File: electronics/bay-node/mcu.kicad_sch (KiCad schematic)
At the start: 15 parts, among them SW1 RESET, SW2 BOOT, U3 ESP32-S3-MINI-1-N8

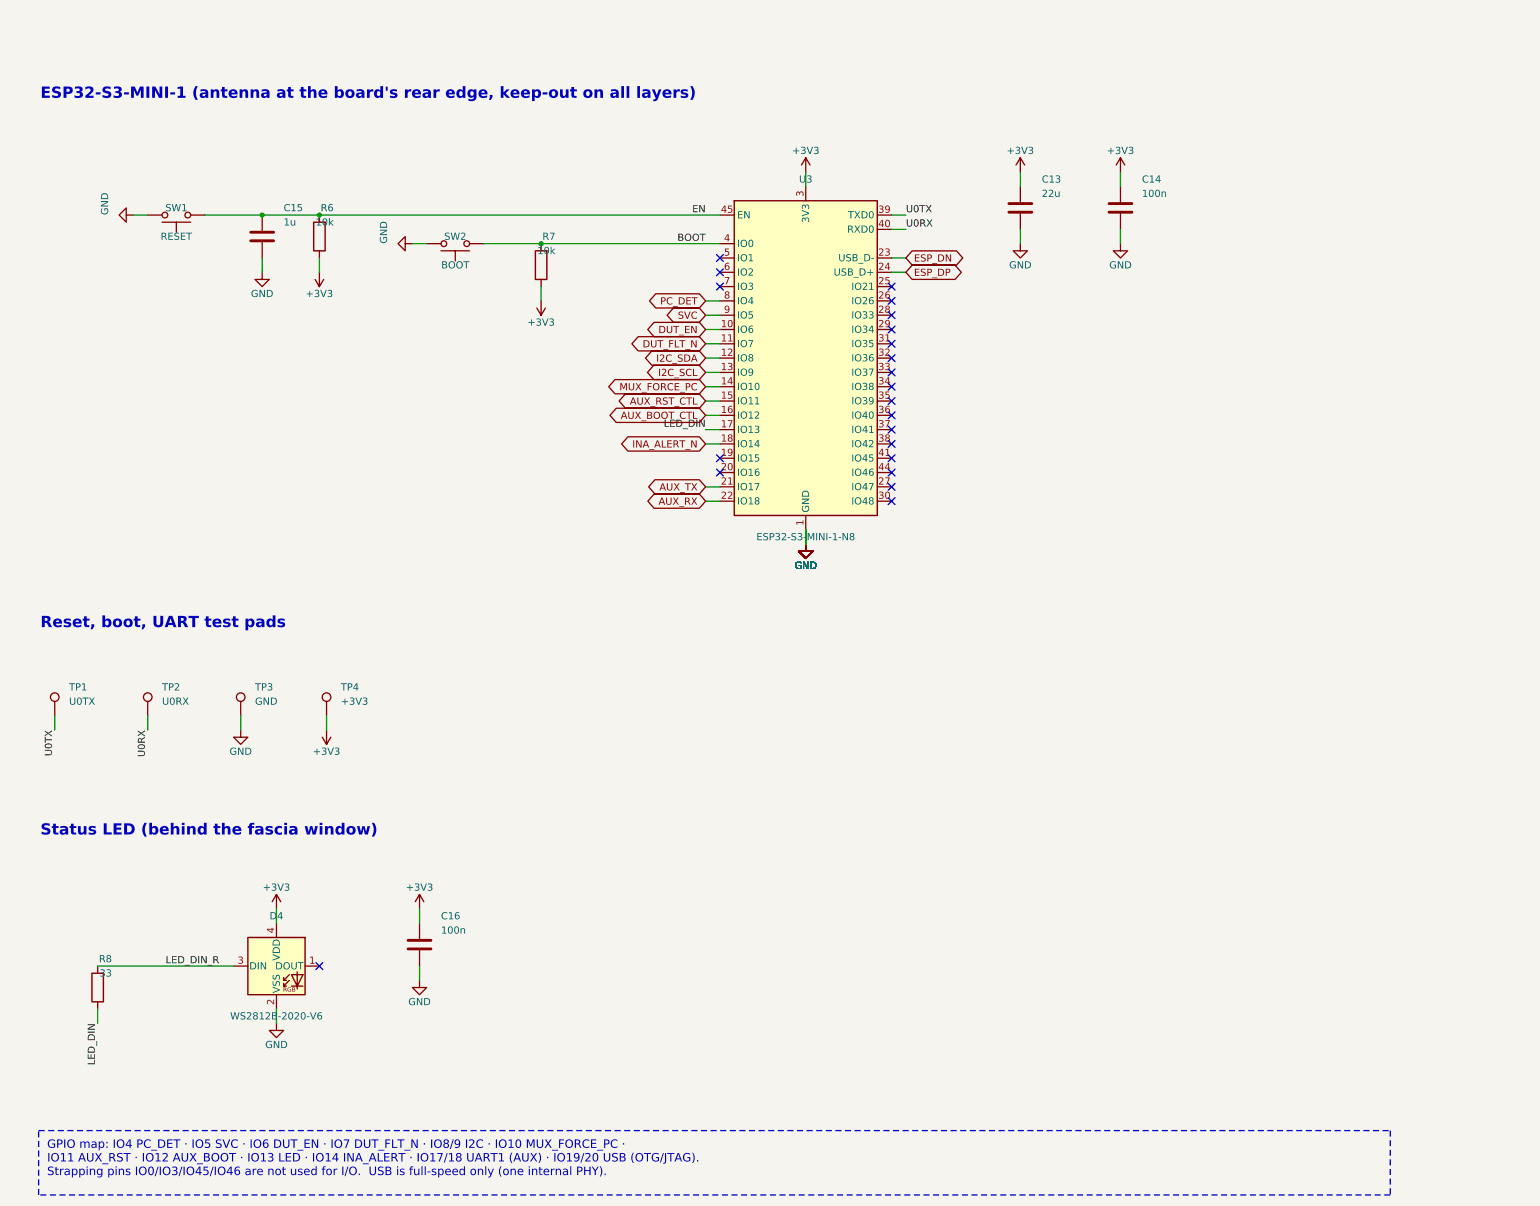
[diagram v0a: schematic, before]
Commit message: Boards v0.2: LMR51635 buck, JST PH, drawn schematics, thermal reliefs
Addresses Fabio's review of v0.1.

Bay node (rev 0.2):
- 5 V buck: LMR51635YDDCR (60 V, 3.5 A, synchronous, 1.1 MHz) with a
  3.3 uH FXL0630, 3 x 22 uF out, 2 x 10 uF + 100 nF in, FB 120k/22k
  (5.16 V), EN 1M/100k UVLO (13.5 V on, 10.8 V off). Replaces the
  TPS54360B, its Schottky and compensation network. CIN straddles the
  VIN/GND pins on solid top-side islands with vias to In1 (TI SLUSF64B).
- 24 V in/out on JST PH (carrier notches resized, rack.yaml pwr_y).
- Power nets named along the path: 24V_BUS -> +24V -> +5V -> DUT_5V_SW
  -> shunt -> DUT_5V; the INA226 visibly runs from +3V3.
- Stackup S+GND / GND / PWR / S+GND: In2 carries +5V, +3V3 under the
  ESP32 and a protected 24 V bus strip. Outer GND pours kept (without
  them Freerouting left ~25 connections unrouted).

Power hub (rev 0.2): JST VH input instead of the screw terminal, JST PH
row outputs, eFuse limit 1.6 A (RILIM 7.5k) to protect the 2 A contacts.

Generator:
- eda.py: drawn schematic mode (sch= placement, Sheet.wire/tag/frame,
  rotated/mirrored symbols, automatic junctions, per-island labels and
  checks that no wire touches another net); all seven sheets redrawn.
- pcbgen.py: thermal reliefs on every pour (+ <board>.kicad_dru for
  single spokes on fine pitch), configurable inner layers, per-zone
  deferral, fixed vias, DRC-driven fix-up for isolated GND pads.
- JLC CPL fix for the LMR51635 (270 deg); BOM, cables, viewer, docs.

ERC 0, DRC 0 copper errors, 0 unconnected, schematic parity 0 on both.

Co-Authored-By: Claude Opus 5.5 <noreply@anthropic.com>
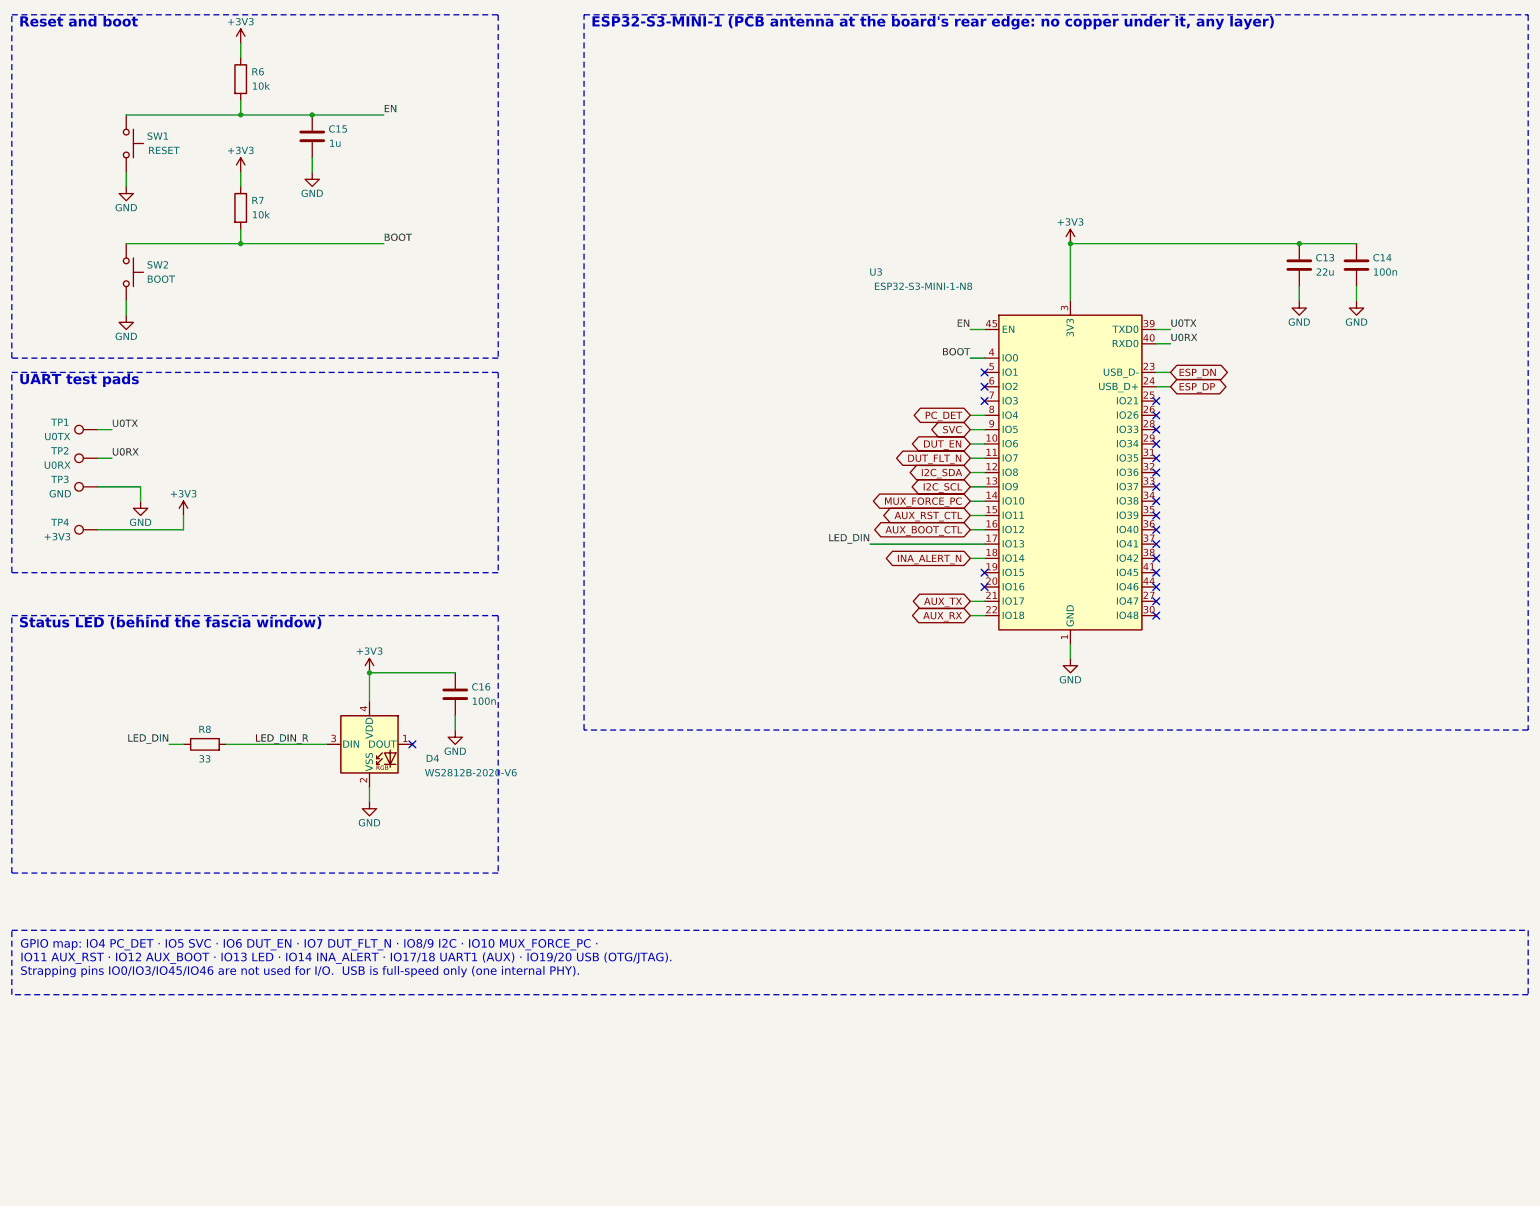
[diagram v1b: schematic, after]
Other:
- note added: "ESP32-S3-MINI-1 (PCB antenna at the board's rear edge: no copper under it, any layer)"
- note added: "Reset and boot"
- note added: "UART test pads"
- note removed: "ESP32-S3-MINI-1 (antenna at the board's rear edge, keep-out on all layers)"
- note removed: "Reset, boot, UART test pads"
- moved on the sheet: C13, C14, C15, C16, D4, R6, R7, R8, SW1, SW2, TP1, TP2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
